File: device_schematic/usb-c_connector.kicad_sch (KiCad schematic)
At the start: 3 parts, among them J1 USB_B

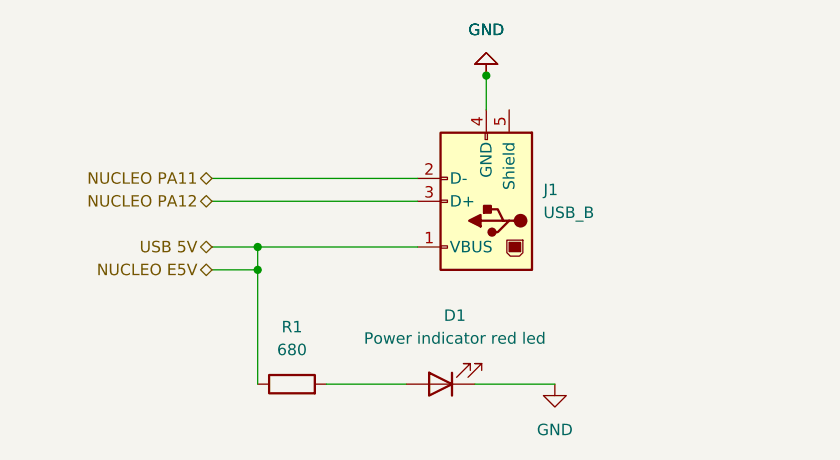
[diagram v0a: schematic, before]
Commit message: Device schematic update
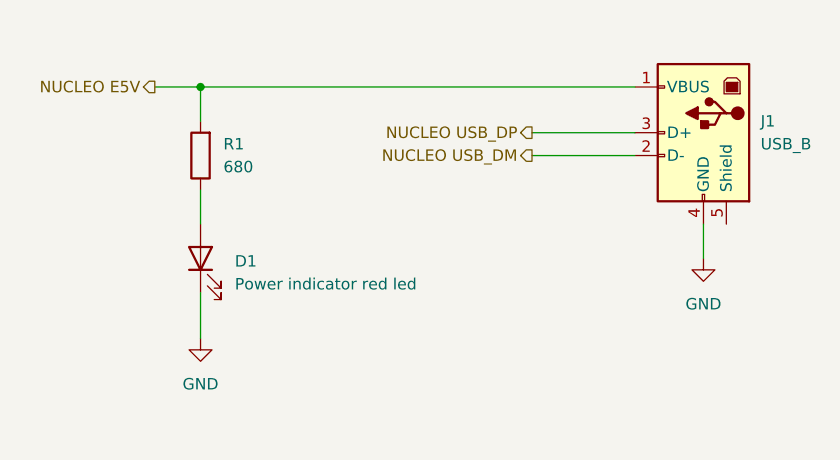
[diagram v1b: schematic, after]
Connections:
- net NUCLEO E5V: now also R1.2; no longer R1.1
- net at D1.2 (A): now also R1.1; no longer R1.2
- net NUCLEO PA11 renamed NUCLEO USB_DM
- net NUCLEO PA12 renamed NUCLEO USB_DP
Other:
- moved on the sheet: D1, J1, R1
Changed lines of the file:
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@@
 (kicad_sch (version 20211123) (generator eeschema)
   (paper "A4")
-  (junction (at 132.08 95.25) (diameter 0) (color 0 0 0 0)
+  (junction (at 125.73 74.93) (diameter 0) (color 0 0 0 0)
   )
-  (junction (at 132.08 92.71) (diameter 0) (color 0 0 0 0)
-  )
-  (junction (at 157.48 73.66) (diameter 0) (color 0 0 0 0)
-  )
-  (wire (pts (xy 127 95.25) (xy 132.08 95.25))
+  (wire (pts (xy 162.56 82.55) (xy 173.99 82.55))
     (stroke (width 0) (type default) (color 0 0 0 0))
   )
-  (wire (pts (xy 127 85.09) (xy 149.86 85.09))
+  (wire (pts (xy 125.73 97.79) (xy 125.73 102.87))
     (stroke (width 0) (type default) (color 0 0 0 0))
   )
-  (wire (pts (xy 132.08 95.25) (xy 132.08 107.95))
+  (wire (pts (xy 125.73 74.93) (xy 125.73 78.74))
     (stroke (width 0) (type default) (color 0 0 0 0))
   )
-  (wire (pts (xy 157.48 73.66) (xy 157.48 77.47))
+  (wire (pts (xy 125.73 86.36) (xy 125.73 90.17))
     (stroke (width 0) (type default) (color 0 0 0 0))
   )
-  (wire (pts (xy 127 92.71) (xy 132.08 92.71))
+  (wire (pts (xy 181.61 90.17) (xy 181.61 93.98))
     (stroke (width 0) (type default) (color 0 0 0 0))
   )
-  (wire (pts (xy 139.7 107.95) (xy 148.59 107.95))
+  (wire (pts (xy 162.56 80.01) (xy 173.99 80.01))
     (stroke (width 0) (type default) (color 0 0 0 0))
   )
-  (wire (pts (xy 132.08 92.71) (xy 132.08 95.25))
+  (wire (pts (xy 125.73 74.93) (xy 173.99 74.93))
     (stroke (width 0) (type default) (color 0 0 0 0))
   )
-  (wire (pts (xy 132.08 92.71) (xy 149.86 92.71))
+  (wire (pts (xy 120.65 74.93) (xy 125.73 74.93))
     (stroke (width 0) (type default) (color 0 0 0 0))
   )
-  (wire (pts (xy 127 87.63) (xy 149.86 87.63))
-    (stroke (width 0) (type default) (color 0 0 0 0))
-  )
-  (wire (pts (xy 156.21 107.95) (xy 165.1 107.95))
-    (stroke (width 0) (type default) (color 0 0 0 0))
-  )
-  (hierarchical_label "NUCLEO PA12" (shape bidirectional) (at 127 87.63 180)
+  (hierarchical_label "NUCLEO USB_DM" (shape output) (at 162.56 82.55 180)
     (effects (font (size 1.27 1.27)) (justify right))
   )
-  (hierarchical_label "USB 5V" (shape bidirectional) (at 127 92.71 180)
+  (hierarchical_label "NUCLEO USB_DP" (shape output) (at 162.56 80.01 180)
     (effects (font (size 1.27 1.27)) (justify right))
   )
-  (hierarchical_label "NUCLEO PA11" (shape bidirectional) (at 127 85.09 180)
+  (hierarchical_label "NUCLEO E5V" (shape output) (at 120.65 74.93 180)
     (effects (font (size 1.27 1.27)) (justify right))
   )
-  (hierarchical_label "NUCLEO E5V" (shape bidirectional) (at 127 95.25 180)
-    (effects (font (size 1.27 1.27)) (justify right))
-  )
-  (symbol (lib_id "Device:R") (at 135.89 107.95 90) (unit 1)
+  (symbol (lib_id "Device:R") (at 125.73 82.55 180) (unit 1)
     (in_bom yes) (on_board yes) (fields_autoplaced)
-    (property "Reference" "R1" (id 0) (at 135.89 101.6 90))
-    (property "Value" "680" (id 1) (at 135.89 104.14 90))
-    (property "Footprint" "" (id 2) (at 135.89 109.728 90)
+    (property "Reference" "R1" (id 0) (at 128.27 81.2799 0)
+      (effects (font (size 1.27 1.27)) (justify right))
+    )
+    (property "Value" "680" (id 1) (at 128.27 83.8199 0)
+      (effects (font (size 1.27 1.27)) (justify right))
+    )
+    (property "Footprint" "" (id 2) (at 127.508 82.55 90)
       (effects (font (size 1.27 1.27)) hide)
     )
-    (property "Datasheet" "~" (id 3) (at 135.89 107.95 0)
+    (property "Datasheet" "~" (id 3) (at 125.73 82.55 0)
       (effects (font (size 1.27 1.27)) hide)
     )
@@
     (pin "2")
   )
-  (symbol (lib_id "Device:LED") (at 152.4 107.95 180) (unit 1)
+  (symbol (lib_id "Device:LED") (at 125.73 93.98 90) (unit 1)
     (in_bom yes) (on_board yes) (fields_autoplaced)
-    (property "Reference" "D1" (id 0) (at 153.9875 100.33 0))
-    (property "Value" "Power indicator red led" (id 1) (at 153.9875 102.87 0))
-    (property "Footprint" "" (id 2) (at 152.4 107.95 0)
+    (property "Reference" "D1" (id 0) (at 129.54 94.2974 90)
+      (effects (font (size 1.27 1.27)) (justify right))
+    )
+    (property "Value" "Power indicator red led" (id 1) (at 129.54 96.8374 90)
+      (effects (font (size 1.27 1.27)) (justify right))
+    )
+    (property "Footprint" "" (id 2) (at 125.73 93.98 0)
       (effects (font (size 1.27 1.27)) hide)
     )
-    (property "Datasheet" "~" (id 3) (at 152.4 107.95 0)
+    (property "Datasheet" "~" (id 3) (at 125.73 93.98 0)
       (effects (font (size 1.27 1.27)) hide)
     )
@@
     (pin "2")
   )
-  (symbol (lib_id "power:GND") (at 157.48 73.66 180) (unit 1)
+  (symbol (lib_id "Connector:USB_B") (at 181.61 80.01 0) (mirror y) (unit 1)
     (in_bom yes) (on_board yes) (fields_autoplaced)
-    (property "Reference" "#PWR?" (id 0) (at 157.48 67.31 0)
+    (property "Reference" "J1" (id 0) (at 187.96 78.7399 0)
+      (effects (font (size 1.27 1.27)) (justify right))
+    )
+    (property "Value" "USB_B" (id 1) (at 187.96 81.2799 0)
+      (effects (font (size 1.27 1.27)) (justify right))
+    )
+    (property "Footprint" "" (id 2) (at 177.8 81.28 0)
       (effects (font (size 1.27 1.27)) hide)
     )
-    (property "Value" "GND" (id 1) (at 157.48 68.58 0))
-    (property "Footprint" "" (id 2) (at 157.48 73.66 0)
-      (effects (font (size 1.27 1.27)) hide)
-    )
-    (property "Datasheet" "" (id 3) (at 157.48 73.66 0)
-      (effects (font (size 1.27 1.27)) hide)
-    )
-    (pin "1")
-  )
-  (symbol (lib_id "Connector:USB_B") (at 157.48 87.63 180) (unit 1)
-    (in_bom yes) (on_board yes) (fields_autoplaced)
-    (property "Reference" "J1" (id 0) (at 163.83 86.3599 0)
-      (effects (font (size 1.27 1.27)) (justify right))
-    )
-    (property "Value" "USB_B" (id 1) (at 163.83 88.8999 0)
-      (effects (font (size 1.27 1.27)) (justify right))
-    )
-    (property "Footprint" "" (id 2) (at 153.67 86.36 0)
-      (effects (font (size 1.27 1.27)) hide)
-    )
-    (property "Datasheet" " ~" (id 3) (at 153.67 86.36 0)
+    (property "Datasheet" " ~" (id 3) (at 177.8 81.28 0)
       (effects (font (size 1.27 1.27)) hide)
     )
@@
     (pin "5")
   )
-  (symbol (lib_id "power:GND") (at 157.48 73.66 180) (unit 1)
+  (symbol (lib_id "power:GND") (at 181.61 93.98 0) (unit 1)
     (in_bom yes) (on_board yes) (fields_autoplaced)
-    (property "Reference" "#PWR?" (id 0) (at 157.48 67.31 0)
+    (property "Reference" "#PWR?" (id 0) (at 181.61 100.33 0)
       (effects (font (size 1.27 1.27)) hide)
     )
-    (property "Value" "GND" (id 1) (at 157.48 68.58 0))
-    (property "Footprint" "" (id 2) (at 157.48 73.66 0)
+    (property "Value" "GND" (id 1) (at 181.61 99.06 0))
+    (property "Footprint" "" (id 2) (at 181.61 93.98 0)
       (effects (font (size 1.27 1.27)) hide)
     )
-    (property "Datasheet" "" (id 3) (at 157.48 73.66 0)
+    (property "Datasheet" "" (id 3) (at 181.61 93.98 0)
       (effects (font (size 1.27 1.27)) hide)
     )
     (pin "1")
   )
-  (symbol (lib_id "power:GND") (at 165.1 107.95 0) (unit 1)
+  (symbol (lib_id "power:GND") (at 125.73 102.87 0) (unit 1)
     (in_bom yes) (on_board yes) (fields_autoplaced)
-    (property "Reference" "#PWR?" (id 0) (at 165.1 114.3 0)
+    (property "Reference" "#PWR?" (id 0) (at 125.73 109.22 0)
       (effects (font (size 1.27 1.27)) hide)
     )
-    (property "Value" "GND" (id 1) (at 165.1 113.03 0))
-    (property "Footprint" "" (id 2) (at 165.1 107.95 0)
+    (property "Value" "GND" (id 1) (at 125.73 107.95 0))
+    (property "Footprint" "" (id 2) (at 125.73 102.87 0)
       (effects (font (size 1.27 1.27)) hide)
     )
-    (property "Datasheet" "" (id 3) (at 165.1 107.95 0)
+    (property "Datasheet" "" (id 3) (at 125.73 102.87 0)
       (effects (font (size 1.27 1.27)) hide)
     )
